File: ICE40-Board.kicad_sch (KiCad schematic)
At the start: 82 parts, among them SW1 SW_Push, U1 ADP1712AUJZ-3.3, U10 FT4222HQ, U11 74LS125, U12 74LS126, U2 ADP1712AUJZ-2.5, U3 ADP1712AUJZ-1.2, U4 Barrel_Jack, U5 W25X20CLSNIG, U6 USB_C_Receptacle_USB2.0, U7 ICE40HX4K-TQ144, U8 W25X20CLSNIG, U9 SIT2001BI-S2-33E-25.000000G

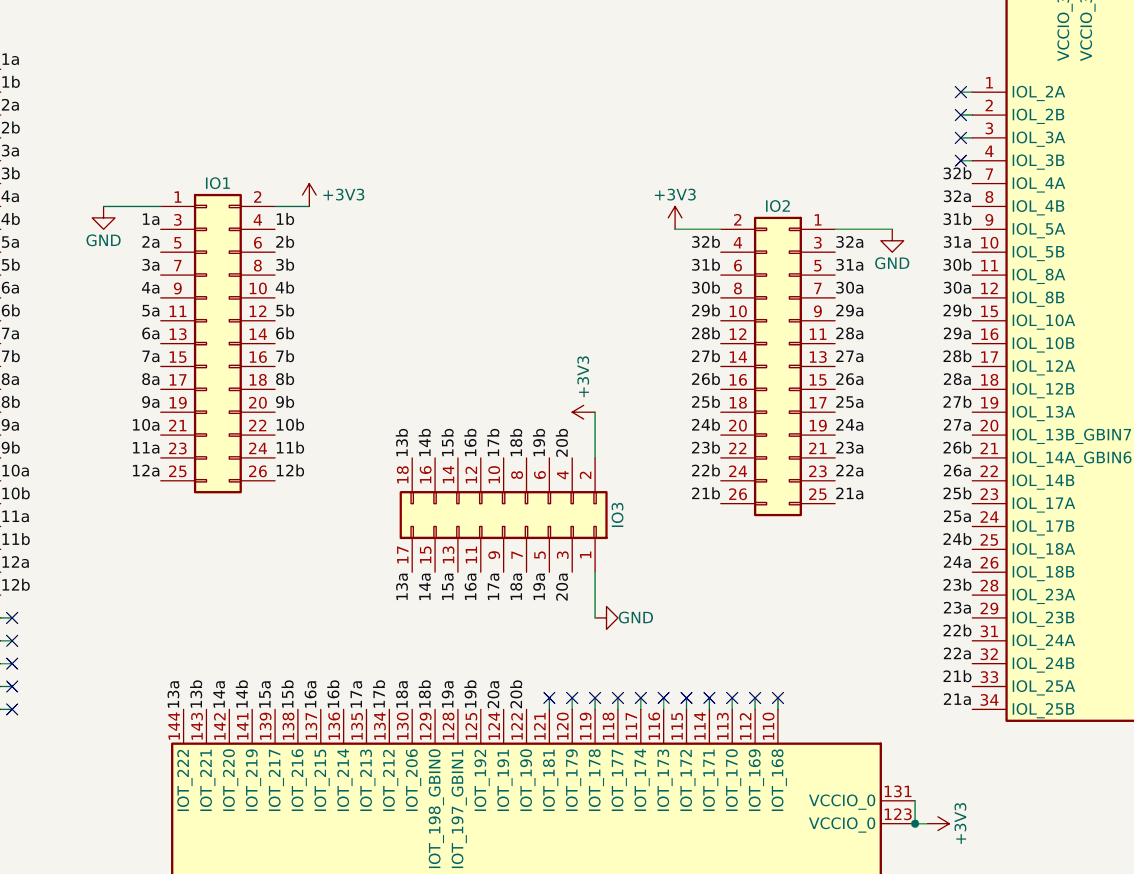
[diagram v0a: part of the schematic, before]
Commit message: No DRC errors, board fully routed
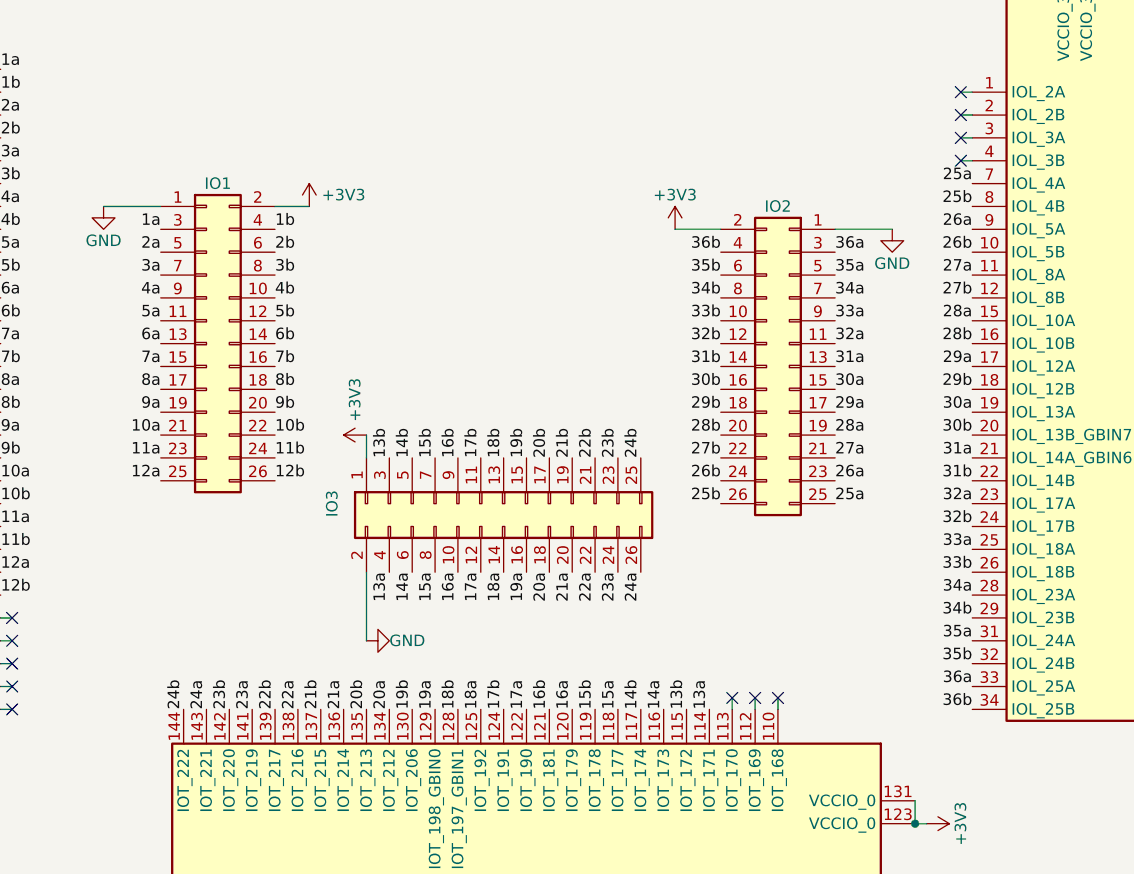
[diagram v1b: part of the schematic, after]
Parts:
- IO3: footprint Connector_PinHeader_2.00mm:PinHeader_2x09_P2.00mm_Vertical -> Connector_PinHeader_2.54mm:PinHeader_2x13_P2.54mm_Vertical; symbol Connector_Generic:Conn_02x09_Odd_Even -> Connector_Generic:Conn_02x13_Odd_Even
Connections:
- net +3V3: now also IO3.1 (Pin_1); no longer IO3.2 (Pin_2)
- net 13a: now also IO3.4 (Pin_4), U7.114 (IOT_171); no longer IO3.17 (Pin_17), U7.144 (IOT_222)
- net 13b: now also IO3.3 (Pin_3), U7.115 (IOT_172); no longer IO3.18 (Pin_18), U7.143 (IOT_221)
- net 14a: now also IO3.6 (Pin_6), U7.116 (IOT_173); no longer IO3.15 (Pin_15), U7.142 (IOT_220)
- net 14b: now also IO3.5 (Pin_5), U7.117 (IOT_174); no longer IO3.16 (Pin_16), U7.141 (IOT_219)
- net 15a: now also IO3.8 (Pin_8), U7.118 (IOT_177); no longer IO3.13 (Pin_13), U7.139 (IOT_217)
- net 15b: now also IO3.7 (Pin_7), U7.119 (IOT_178); no longer IO3.14 (Pin_14), U7.138 (IOT_216)
- net 16a: now also IO3.10 (Pin_10), U7.120 (IOT_179); no longer IO3.11 (Pin_11), U7.137 (IOT_215)
- net 16b: now also IO3.9 (Pin_9), U7.121 (IOT_181); no longer IO3.12 (Pin_12), U7.136 (IOT_214)
- net 17a: now also IO3.12 (Pin_12), U7.122 (IOT_190); no longer IO3.9 (Pin_9), U7.135 (IOT_213)
- net 17b: now also IO3.11 (Pin_11), U7.124 (IOT_191); no longer IO3.10 (Pin_10), U7.134 (IOT_212)
- net 18a: now also IO3.14 (Pin_14), U7.125 (IOT_192); no longer IO3.7 (Pin_7), U7.130 (IOT_206)
- net 18b: now also IO3.13 (Pin_13), U7.128 (IOT_197_GBIN1); no longer IO3.8 (Pin_8), U7.129 (IOT_198_GBIN0)
- net 19a: now also IO3.16 (Pin_16), U7.129 (IOT_198_GBIN0); no longer IO3.5 (Pin_5), U7.128 (IOT_197_GBIN1)
- net 19b: now also IO3.15 (Pin_15), U7.130 (IOT_206); no longer IO3.6 (Pin_6), U7.125 (IOT_192)
- net 20a: now also IO3.18 (Pin_18), U7.134 (IOT_212); no longer IO3.3 (Pin_3), U7.124 (IOT_191)
- net 20b: now also IO3.17 (Pin_17), U7.135 (IOT_213); no longer IO3.4 (Pin_4), U7.122 (IOT_190)
- net 21a: now also IO3.20 (Pin_20), U7.136 (IOT_214); no longer IO2.25 (Pin_25), U7.34 (IOL_25B)
- net 21b: now also IO3.19 (Pin_19), U7.137 (IOT_215); no longer IO2.26 (Pin_26), U7.33 (IOL_25A)
- net 22a: now also IO3.22 (Pin_22), U7.138 (IOT_216); no longer IO2.23 (Pin_23), U7.32 (IOL_24B)
- net 22b: now also IO3.21 (Pin_21), U7.139 (IOT_217); no longer IO2.24 (Pin_24), U7.31 (IOL_24A)
- net 23a: now also IO3.24 (Pin_24), U7.141 (IOT_219); no longer IO2.21 (Pin_21), U7.29 (IOL_23B)
- net 23b: now also IO3.23 (Pin_23), U7.142 (IOT_220); no longer IO2.22 (Pin_22), U7.28 (IOL_23A)
- net 24a: now also IO3.26 (Pin_26), U7.143 (IOT_221); no longer IO2.19 (Pin_19), U7.26 (IOL_18B)
- net 24b: now also IO3.25 (Pin_25), U7.144 (IOT_222); no longer IO2.20 (Pin_20), U7.25 (IOL_18A)
- net 25a: now also IO2.25 (Pin_25), U7.7 (IOL_4A); no longer IO2.17 (Pin_17), U7.24 (IOL_17B)
- net 25b: now also IO2.26 (Pin_26), U7.8 (IOL_4B); no longer IO2.18 (Pin_18), U7.23 (IOL_17A)
- net 26a: now also IO2.23 (Pin_23), U7.9 (IOL_5A); no longer IO2.15 (Pin_15), U7.22 (IOL_14B)
- net 26b: now also IO2.24 (Pin_24), U7.10 (IOL_5B); no longer IO2.16 (Pin_16), U7.21 (IOL_14A_GBIN6)
- net 27a: now also IO2.21 (Pin_21), U7.11 (IOL_8A); no longer IO2.13 (Pin_13), U7.20 (IOL_13B_GBIN7)
- net 27b: now also IO2.22 (Pin_22), U7.12 (IOL_8B); no longer IO2.14 (Pin_14), U7.19 (IOL_13A)
- net 28a: now also IO2.19 (Pin_19), U7.15 (IOL_10A); no longer IO2.11 (Pin_11), U7.18 (IOL_12B)
- net 28b: now also IO2.20 (Pin_20), U7.16 (IOL_10B); no longer IO2.12 (Pin_12), U7.17 (IOL_12A)
- net 29a: now also IO2.17 (Pin_17), U7.17 (IOL_12A); no longer IO2.9 (Pin_9), U7.16 (IOL_10B)
- net 29b: now also IO2.18 (Pin_18), U7.18 (IOL_12B); no longer IO2.10 (Pin_10), U7.15 (IOL_10A)
- net 30a: now also IO2.15 (Pin_15), U7.19 (IOL_13A); no longer IO2.7 (Pin_7), U7.12 (IOL_8B)
- net 30b: now also IO2.16 (Pin_16), U7.20 (IOL_13B_GBIN7); no longer IO2.8 (Pin_8), U7.11 (IOL_8A)
- net 31a: now also IO2.13 (Pin_13), U7.21 (IOL_14A_GBIN6); no longer IO2.5 (Pin_5), U7.10 (IOL_5B)
- net 31b: now also IO2.14 (Pin_14), U7.22 (IOL_14B); no longer IO2.6 (Pin_6), U7.9 (IOL_5A)
- net 32a: now also IO2.11 (Pin_11), U7.23 (IOL_17A); no longer IO2.3 (Pin_3), U7.8 (IOL_4B)
- net 32b: now also IO2.12 (Pin_12), U7.24 (IOL_17B); no longer IO2.4 (Pin_4), U7.7 (IOL_4A)
- net GND: now also IO3.2 (Pin_2); no longer IO3.1 (Pin_1)
- new net 33a: IO2.9 (Pin_9), U7.25 (IOL_18A)
- new net 33b: IO2.10 (Pin_10), U7.26 (IOL_18B)
- new net 34a: IO2.7 (Pin_7), U7.28 (IOL_23A)
- new net 34b: IO2.8 (Pin_8), U7.29 (IOL_23B)
- new net 35a: IO2.5 (Pin_5), U7.31 (IOL_24A)
- new net 35b: IO2.6 (Pin_6), U7.32 (IOL_24B)
- new net 36a: IO2.3 (Pin_3), U7.33 (IOL_25A)
- new net 36b: IO2.4 (Pin_4), U7.34 (IOL_25B)
- no-connect marks 40 -> 32
